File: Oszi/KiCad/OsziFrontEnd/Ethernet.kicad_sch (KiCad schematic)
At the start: 1 part, among them U5 W5500

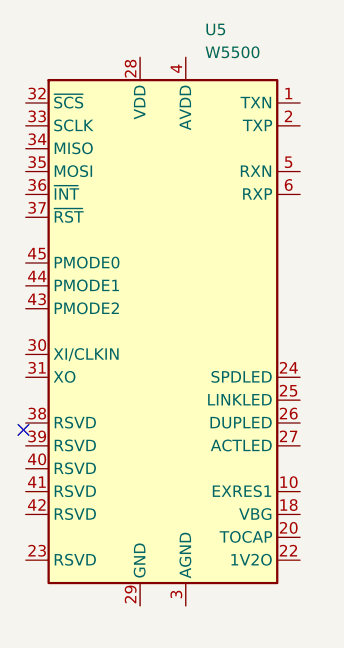
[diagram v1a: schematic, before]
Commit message: jetzt git
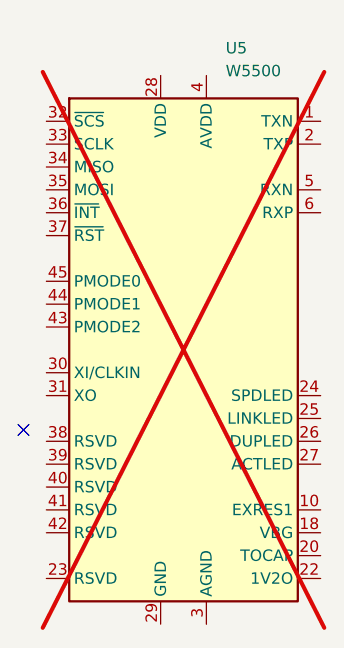
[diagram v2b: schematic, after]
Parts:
- U5: now not fitted; now left out of the parts list
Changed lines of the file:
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@@
 	(symbol
 		(lib_id "Interface_Ethernet:W5500")
-		(at 87.884 67.818 0)
+		(at 90.17 69.85 0)
 		(unit 1)
-		(exclude_from_sim no)
-		(in_bom yes)
+		(exclude_from_sim yes)
+		(in_bom no)
 		(on_board no)
-		(dnp no)
+		(dnp yes)
 		(fields_autoplaced yes)
 		(property "Reference" "U5"
-			(at 92.5673 34.29 0)
+			(at 94.8533 36.322 0)
 			(effects
 				(font
@@
 		)
 		(property "Value" "W5500"
-			(at 92.5673 36.83 0)
+			(at 94.8533 38.862 0)
 			(effects
 				(font
@@
 		)
 		(property "Footprint" "Package_QFP:LQFP-48_7x7mm_P0.5mm"
-			(at 87.884 25.908 0)
+			(at 90.17 27.94 0)
 			(effects
 				(font
@@
 		)
 		(property "Datasheet" "http://wizwiki.net/wiki/lib/exe/fetch.php/products:w5500:w5500_ds_v109e.pdf"
-			(at 87.884 42.418 0)
+			(at 90.17 44.45 0)
 			(effects
 				(font
@@
 		)
 		(property "Description" "10/100Mb SPI Ethernet controller with TCP/IP stack, LQFP-48"
-			(at 87.884 67.818 0)
+			(at 90.17 69.85 0)
 			(effects
 				(font
